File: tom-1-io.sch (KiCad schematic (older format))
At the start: 4 parts, among them J1 Conn_02x06_Counter_Clockwise, J3 Conn_02x06_Counter_Clockwise, U1 74LS377, U5 74LS377

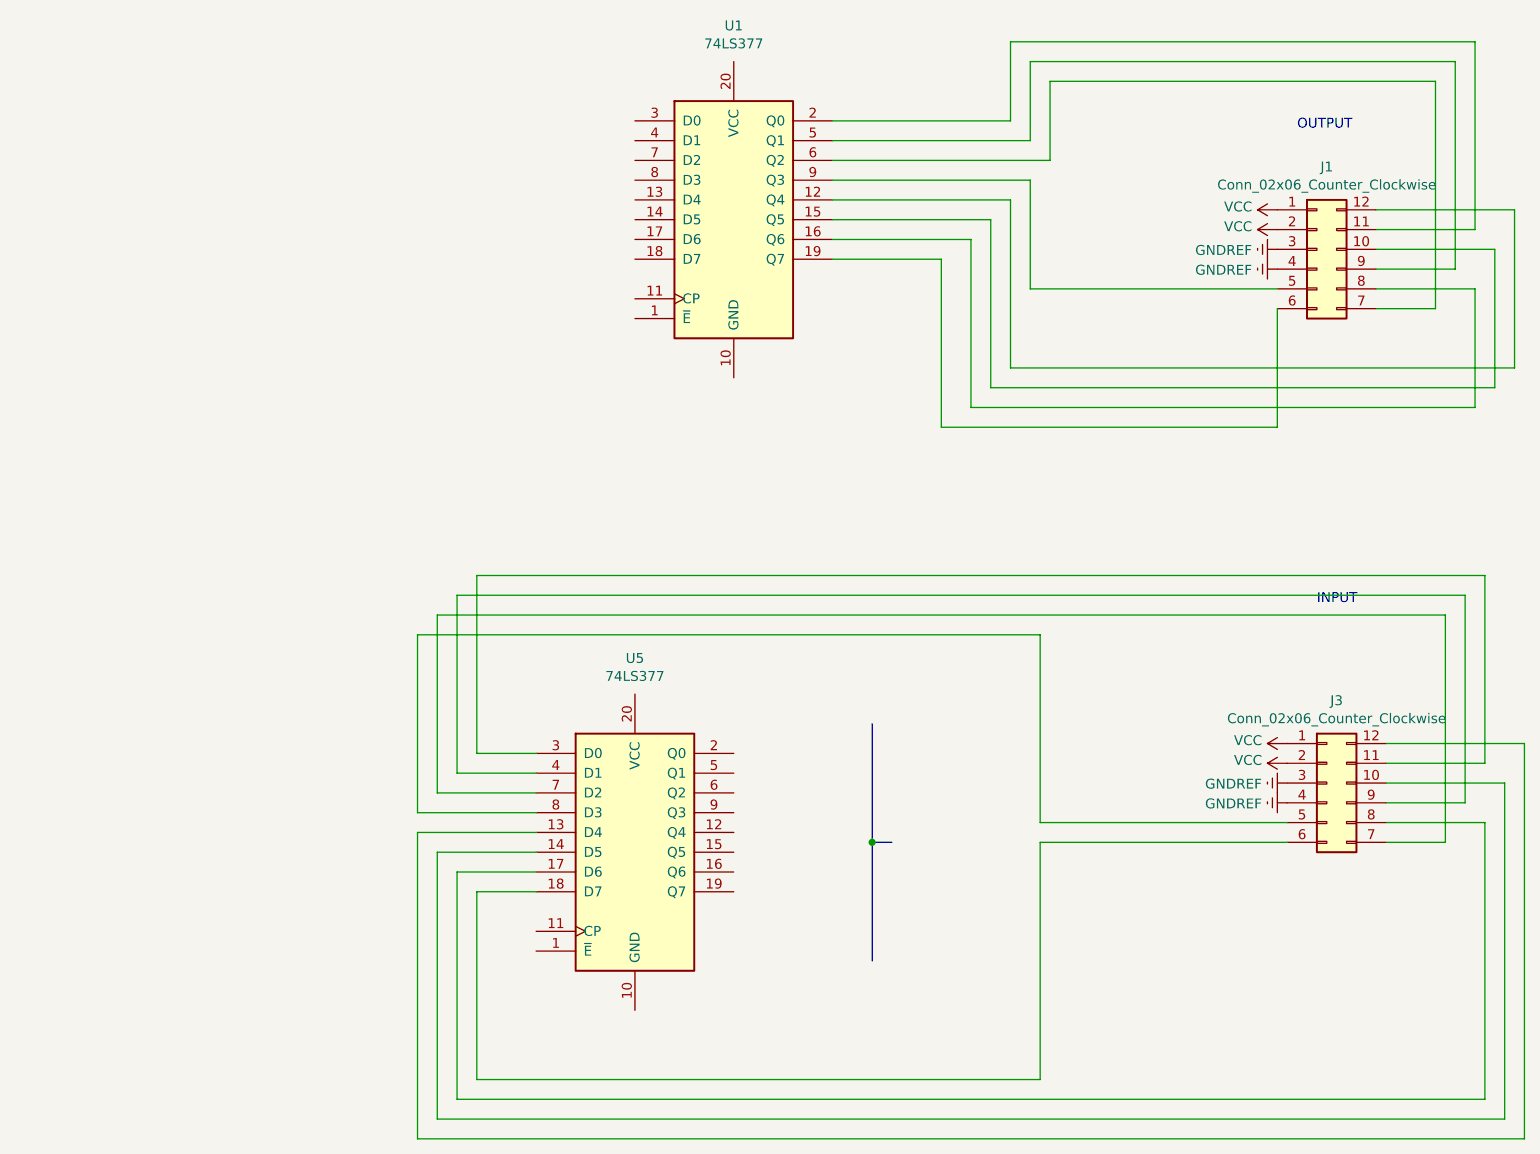
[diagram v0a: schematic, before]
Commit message: Next level
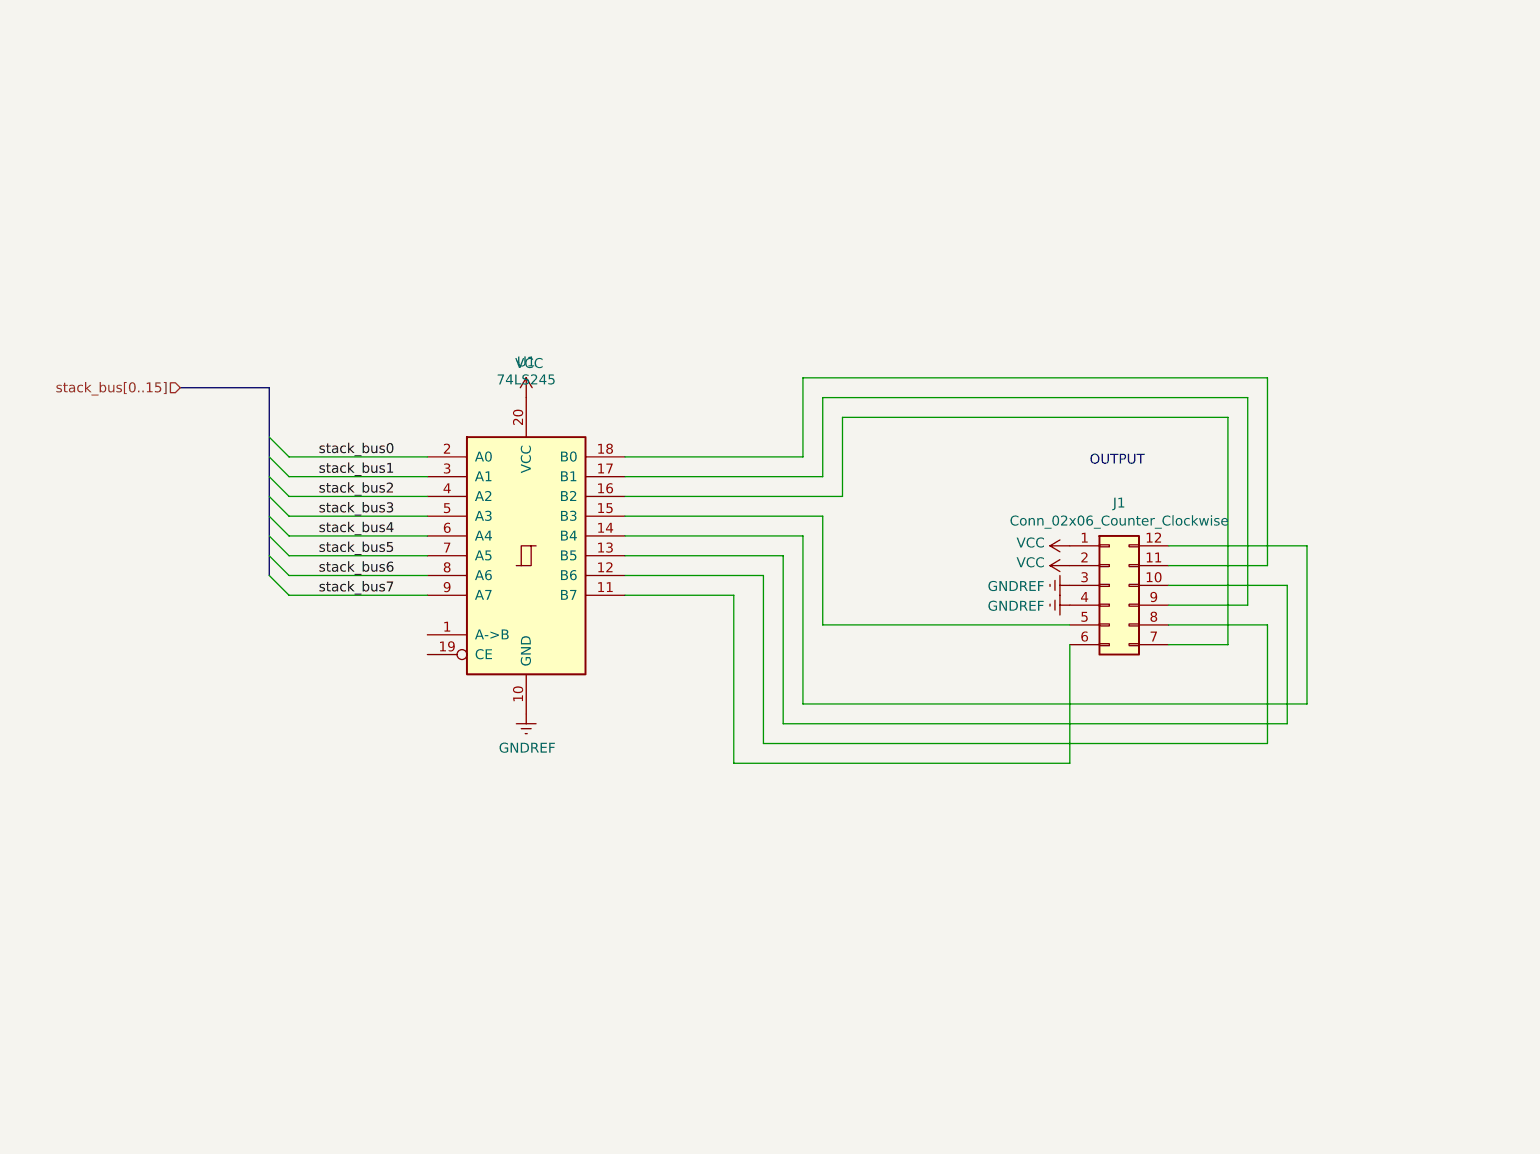
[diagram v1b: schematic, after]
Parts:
- removed J3: Conn_02x06_Counter_Clockwise, Connector_PinSocket_2.54mm:PinSocket_2x06_P2.54mm_Vertical, symbol Connector_Generic:Conn_02x06_Counter_Clockwise
- removed U1, U5: 74LS377, Package_DIP:DIP-20_W7.62mm, symbol 74xx:74LS377
- added U1: 74LS245, Package_DIP:DIP-20_W7.62mm, symbol 74xx:74LS245
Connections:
- net GNDREF: now also U1.10 (GND)
- net VCC: now also U1.20 (VCC)
- net at J1.12 (Pin_12): now also U1.14 (B4)
- net at J1.10 (Pin_10): now also U1.13 (B5)
- net at J1.8 (Pin_8): now also U1.12 (B6)
- net at J1.6 (Pin_6): now also U1.11 (B7)
- net at J1.11 (Pin_11): now also U1.18 (B0)
- net at J1.9 (Pin_9): now also U1.17 (B1)
- net at J1.7 (Pin_7): now also U1.16 (B2)
- net at J1.5 (Pin_5): now also U1.15 (B3)
- new net stack_bus0: U1.2 (A0)
- new net stack_bus1: U1.3 (A1)
- new net stack_bus2: U1.4 (A2)
- new net stack_bus3: U1.5 (A3)
- new net stack_bus4: U1.6 (A4)
- new net stack_bus5: U1.7 (A5)
- new net stack_bus6: U1.8 (A6)
- new net stack_bus7: U1.9 (A7)
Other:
- note removed: "INPUT"
- moved on the sheet: J1
